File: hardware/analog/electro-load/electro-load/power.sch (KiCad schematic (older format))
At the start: 14 parts, among them J2 Jack-DC, U3 NCP1406SNT1G

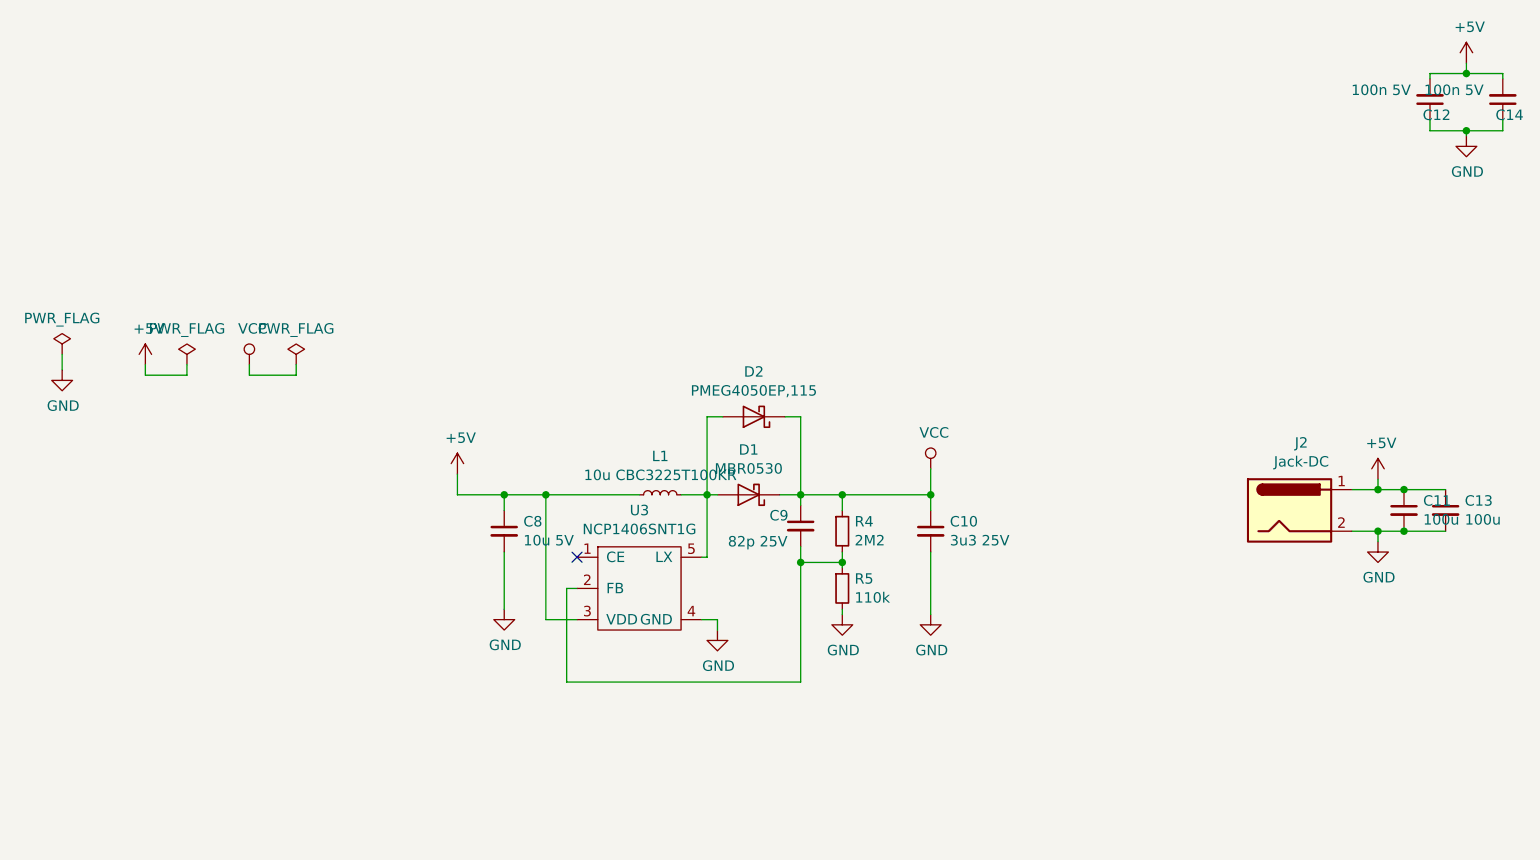
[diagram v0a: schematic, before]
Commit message: HW rev 1 of electronic load PCB.
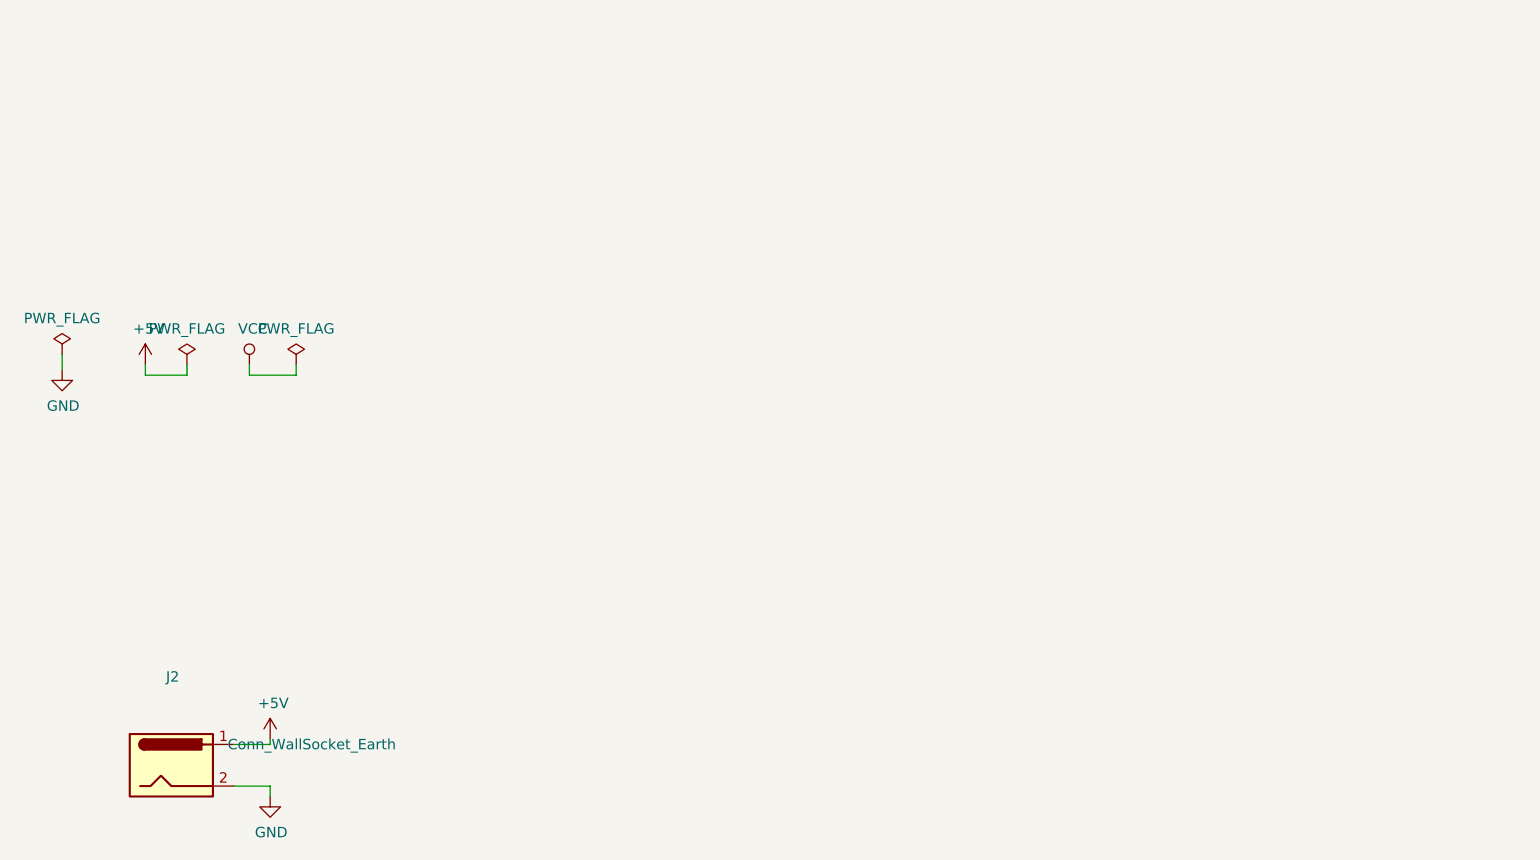
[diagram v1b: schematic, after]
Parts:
- removed C10: 3u3 25V, Capacitor_SMD:C_0805_2012Metric, symbol Device:C_Small
- removed C11, C13: 100u, Capacitor_SMD:CP_Elec_6.3x7.7, symbol Device:C_Small
- removed C12, C14: 100n 5V, Capacitor_SMD:C_0603_1608Metric, symbol Device:C_Small
- removed C8: 10u 5V, Capacitor_SMD:C_0805_2012Metric, symbol Device:C_Small
- removed C9: 82p 25V, Capacitor_SMD:C_0603_1608Metric, symbol Device:C_Small
- removed D1: MBR0530, Diode_SMD:D_SOD-123, symbol Diode:MBR0530
- removed D2: PMEG4050EP,115, athir:SOD128, symbol Diode:MBR0530
- removed L1: 10u CBC3225T100KR, Inductor_SMD:L_1210_3225Metric, symbol Device:L_Small
- removed R4: 2M2, Resistor_SMD:R_0603_1608Metric, symbol Device:R_Small
- removed R5: 110k, Resistor_SMD:R_0603_1608Metric, symbol Device:R_Small
- removed U3: NCP1406SNT1G, Package_TO_SOT_SMD:SOT-23-5, symbol athir:NCP1406SNT1G
- J2: value Jack-DC -> Conn_WallSocket_Earth; footprint Connector_PinHeader_2.54mm:PinHeader_1x02_P2.54mm_Vertical -> athir:230VAC_PLUG
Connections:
- no-connect marks 1 -> 0
